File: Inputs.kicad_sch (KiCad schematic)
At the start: 0 parts

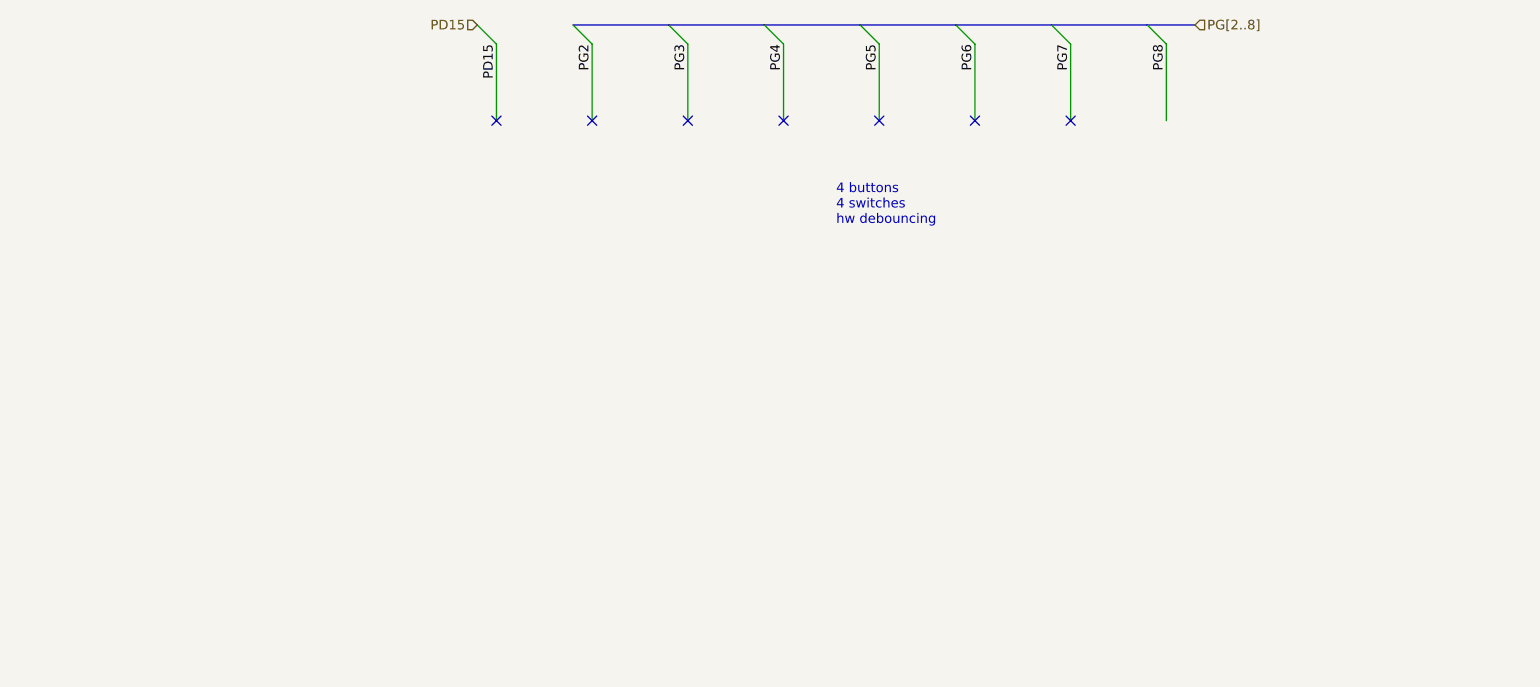
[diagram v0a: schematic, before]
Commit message: basic inputs
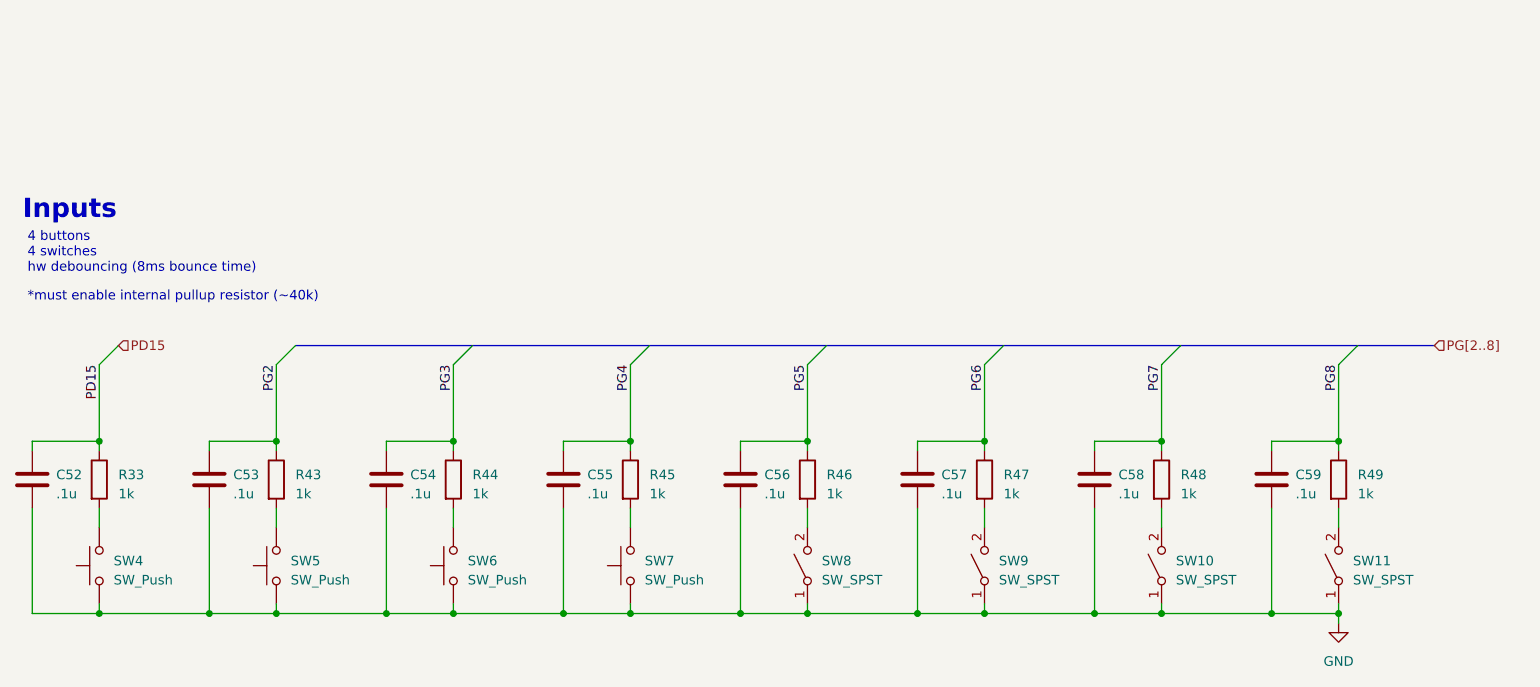
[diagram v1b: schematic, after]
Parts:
- added C52, C53, C54, C55, C56, C57, C58, C59: .1u, symbol Device:C
- added R33, R43, R44, R45, R46, R47, R48, R49: 1k, symbol Device:R
- added SW10, SW11, SW8, SW9: SW_SPST, symbol Switch:SW_SPST
- added SW4, SW5, SW6, SW7: SW_Push, symbol Switch:SW_Push
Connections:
- net PD15: now also C52.1, R33.1
- net PG2: now also C53.1, R43.1
- net PG3: now also C54.1, R44.1
- net PG4: now also C55.1, R45.1
- net PG5: now also C56.1, R46.1
- net PG6: now also C57.1, R47.1
- net PG7: now also C58.1, R48.1
- net PG8: now also C59.1, R49.1
- new net: R48.2, SW10.2 (B)
- new net: R46.2, SW8.2 (B)
- new net: R44.2, SW6.2
- new net: R49.2, SW11.2 (B)
- new net: R45.2, SW7.2
- new net: R33.2, SW4.2
- new net: R47.2, SW9.2 (B)
- new net: R43.2, SW5.2
- new net GND: C52.2, C53.2, C54.2, C55.2, C56.2, C57.2, C58.2, C59.2, SW10.1 (A), SW11.1 (A), SW4.1, SW5.1, SW6.1, SW7.1, SW8.1 (A), SW9.1 (A)
- no-connect marks 7 -> 0
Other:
- note added: "*must enable internal pullup resistor (~40k)"
- note added: "4 buttons 4 switches hw debouncing (8ms bounce time)"
- note added: "Inputs"
- note removed: "4 buttons 4 switches hw debouncing"
